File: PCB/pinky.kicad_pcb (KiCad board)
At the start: 2 copper layers, 134.3 x 87.7 mm, 54 parts, among them SW10 Switch, SW11 Switch, SW12 Switch, SW13 Switch, SW14 Switch, SW15 Switch, SW16 Switch, SW17 Switch, SW18 Switch, SW2 Switch, SW3 Switch, SW5 Switch, SW6 Switch, SW7 Switch, SW8 Switch, SW9 Switch, U1 nice!nano

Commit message: Pulled updates
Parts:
- D1, D10, D11, D12, D13, D14, D15, D16, D17, D2, D4, D5, D6, D7, D8, D9: value D_SOD123 -> D
- JP1, JP10, JP2, JP3, JP4, JP5, JP6, JP7, JP8, JP9: value Jumper -> SDA
- RESET19: value ResetSW -> Val**
- SW10, SW11, SW12, SW13, SW14, SW15, SW16, SW17, SW18, SW2, SW3, SW5, SW6, SW7, SW8, SW9: value Switch -> SW_Kailh_Choc_PG1350

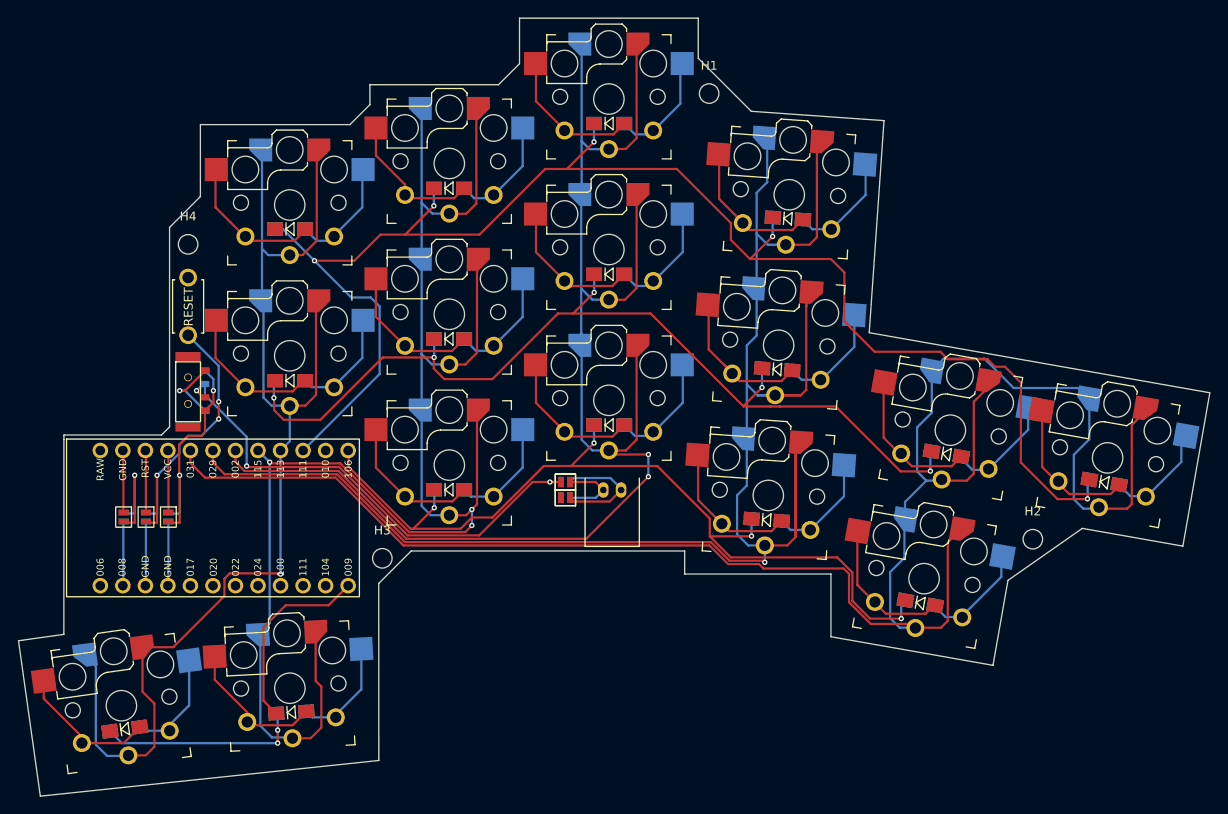
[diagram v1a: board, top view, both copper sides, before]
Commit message: Work in progress on shaping up the edges
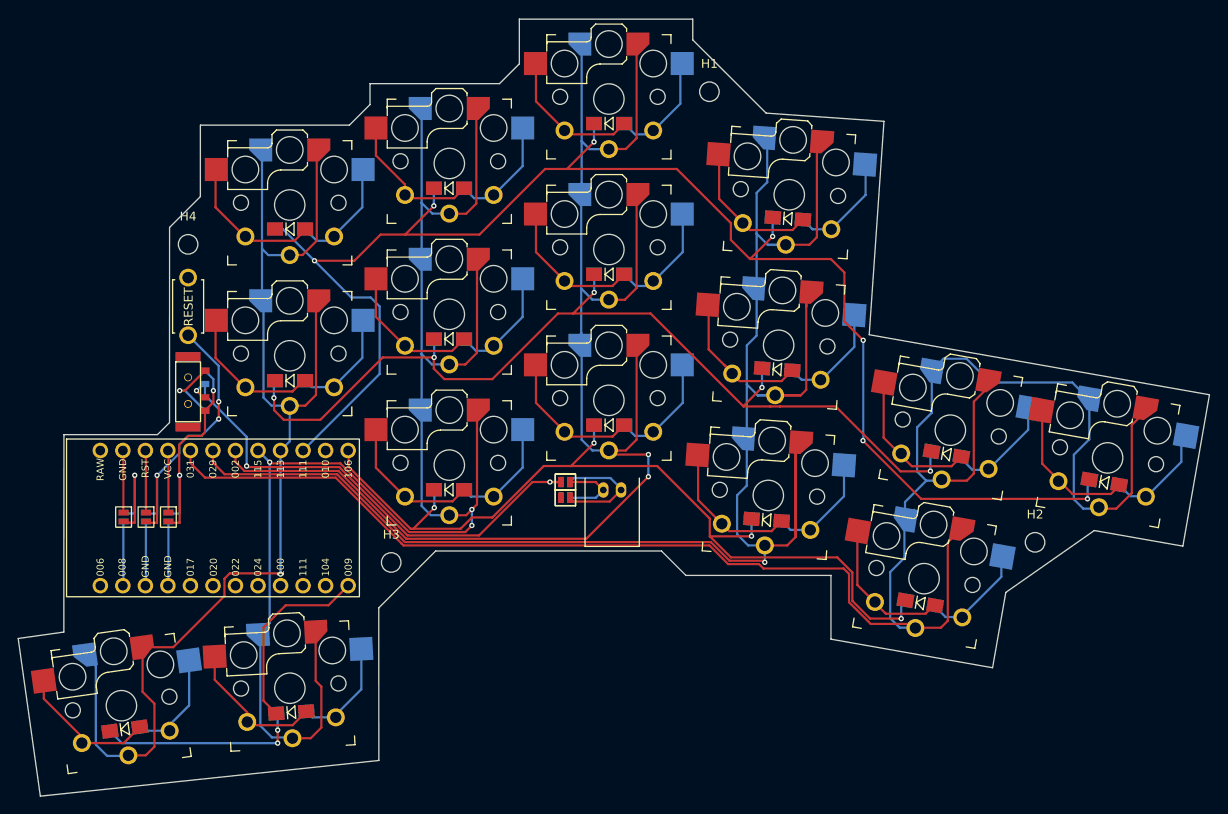
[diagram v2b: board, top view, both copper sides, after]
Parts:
- moved H3 1.10 mm to (128.4, 110.9)
- moved H2 0.43 mm to (201.0, 108.6)
- moved H1 0.21 mm to (164.3, 57.8)
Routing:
- net row_A: track 173.1 -> 173.9 mm, vias 5 -> 7
- net col_E: track 210.0 -> 209.3 mm
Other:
- board size 134.3 x 87.7 mm -> 134.3 x 87.6 mm
